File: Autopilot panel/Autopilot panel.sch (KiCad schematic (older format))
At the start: 21 parts, among them J1 USB_B_Micro, J2 Conn_02x15_Odd_Even, J8 Conn_02x15_Odd_Even, SW1 SW_Push, SW2 SW_Push, SW3 SW_Push, SW4 SW_Push, SW5 SW_Push

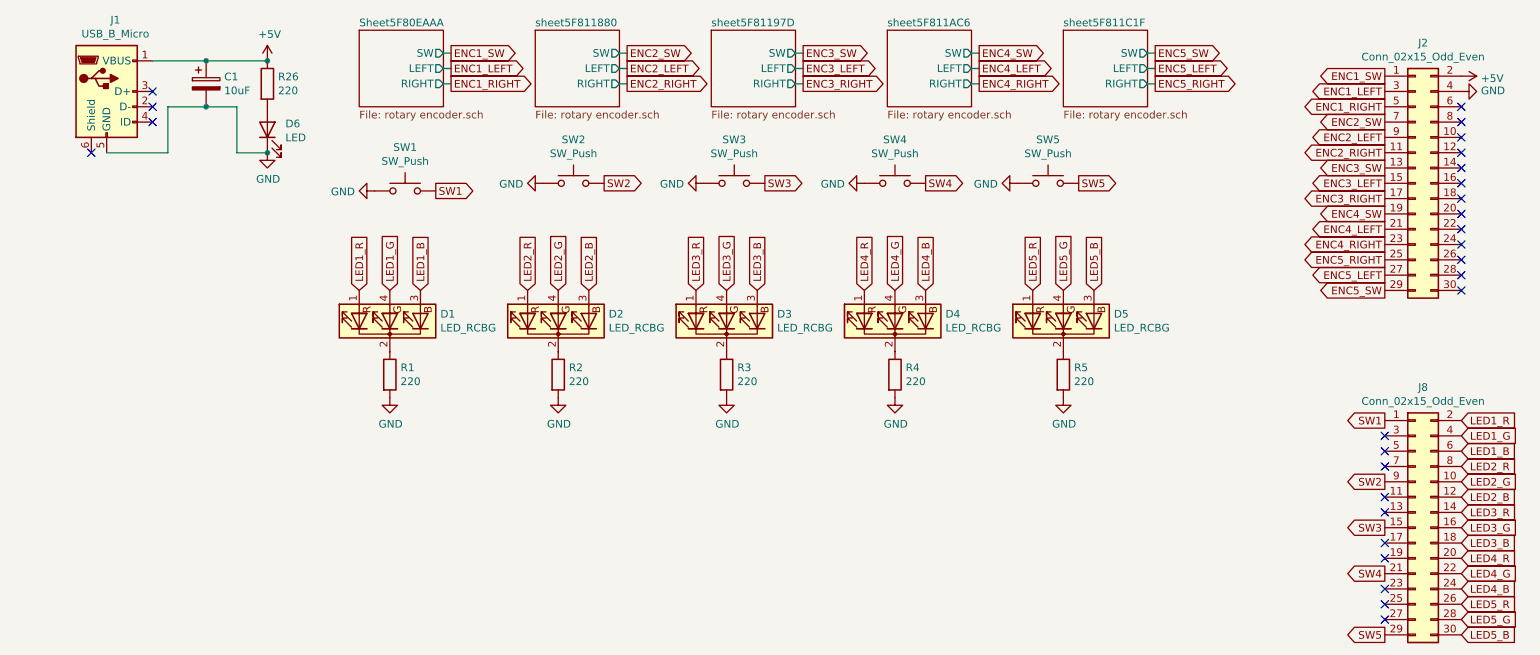
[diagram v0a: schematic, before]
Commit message: Submitted version!
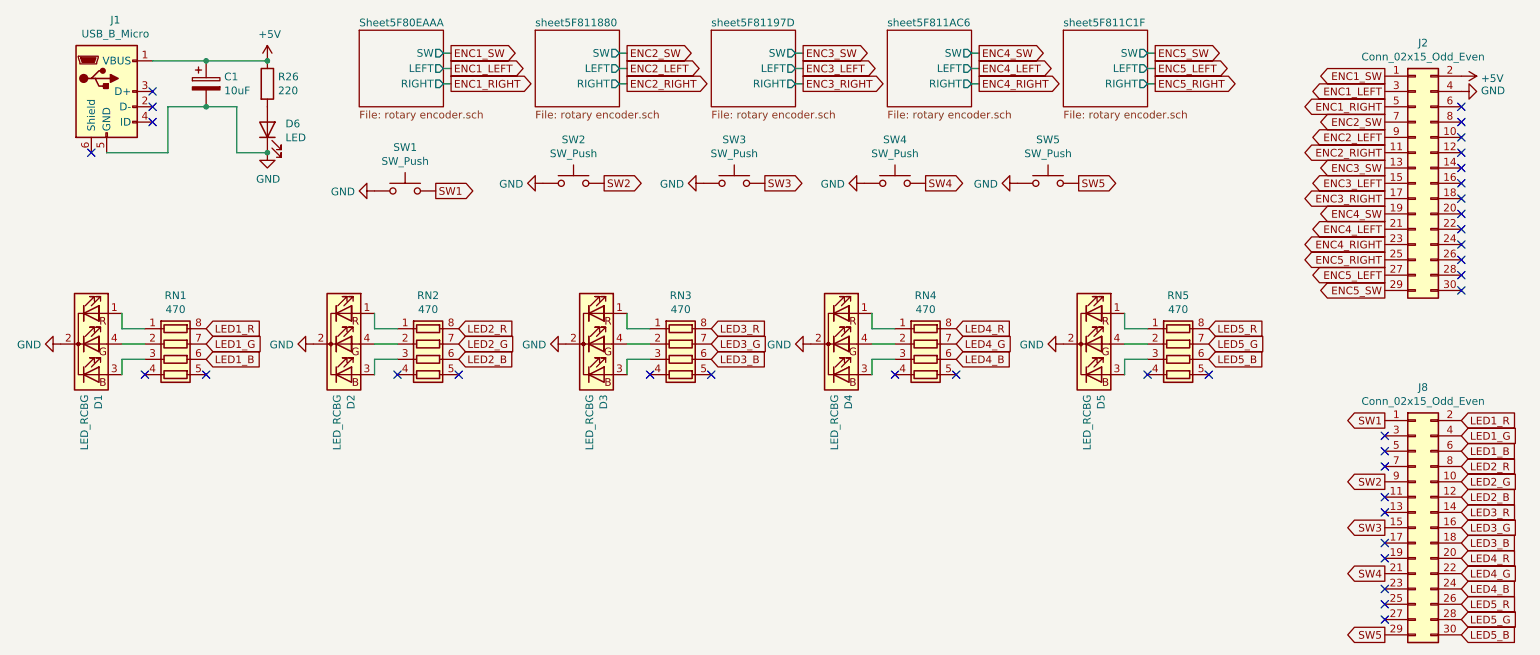
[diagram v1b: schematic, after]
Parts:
- removed R1, R2, R3, R4, R5: 220, Resistor_SMD:R_0805_2012Metric_Pad1.15x1.40mm_HandSolder, symbol Device:R
- added RN1, RN2, RN3, RN4, RN5: 470, Resistor_SMD:R_Array_Convex_4x0603, symbol Device:R_Pack04
- C1: footprint Capacitor_Tantalum_SMD:CP_EIA-3216-18_Kemet-A -> Capacitor_THT:CP_Radial_D5.0mm_P2.00mm
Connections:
- net GND: now also D1.2 (K), D2.2 (K), D3.2 (K), D4.2 (K), D5.2 (K)
- net LED1_B: now also RN1.6 (R3.2); no longer D1.3 (BA)
- net LED1_G: now also RN1.7 (R2.2); no longer D1.4 (GA)
- net LED1_R: now also RN1.8 (R1.2); no longer D1.1 (RA)
- net LED2_B: now also RN2.6 (R3.2); no longer D2.3 (BA)
- net LED2_G: now also RN2.7 (R2.2); no longer D2.4 (GA)
- net LED2_R: now also RN2.8 (R1.2); no longer D2.1 (RA)
- net LED3_B: now also RN3.6 (R3.2); no longer D3.3 (BA)
- net LED3_G: now also RN3.7 (R2.2); no longer D3.4 (GA)
- net LED3_R: now also RN3.8 (R1.2); no longer D3.1 (RA)
- net LED4_B: now also RN4.6 (R3.2); no longer D4.3 (BA)
- net LED4_G: now also RN4.7 (R2.2); no longer D4.4 (GA)
- net LED4_R: now also RN4.8 (R1.2); no longer D4.1 (RA)
- net LED5_B: now also RN5.6 (R3.2); no longer D5.3 (BA)
- net LED5_G: now also RN5.7 (R2.2); no longer D5.4 (GA)
- net LED5_R: now also RN5.8 (R1.2); no longer D5.1 (RA)
- new net: D1.1 (RA), RN1.1 (R1.1)
- new net: D1.3 (BA), RN1.3 (R3.1)
- new net: D1.4 (GA), RN1.2 (R2.1)
- new net: D2.1 (RA), RN2.1 (R1.1)
- new net: D2.3 (BA), RN2.3 (R3.1)
- new net: D2.4 (GA), RN2.2 (R2.1)
- new net: D3.1 (RA), RN3.1 (R1.1)
- new net: D3.3 (BA), RN3.3 (R3.1)
- new net: D3.4 (GA), RN3.2 (R2.1)
- new net: D4.1 (RA), RN4.1 (R1.1)
- new net: D4.3 (BA), RN4.3 (R3.1)
- new net: D4.4 (GA), RN4.2 (R2.1)
- new net: D5.1 (RA), RN5.1 (R1.1)
- new net: D5.3 (BA), RN5.3 (R3.1)
- new net: D5.4 (GA), RN5.2 (R2.1)
- no-connect marks 27 -> 37
